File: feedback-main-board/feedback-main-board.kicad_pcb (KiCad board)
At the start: 4 copper layers, 80 x 64 mm, 88 parts, among them J1 908140508, J2 FLIP, J3 RPT, Q1 MMFTP3401, Q2 MMBT3904, Q3 MMBT3904, Q4 MMBT3904, SW1 SW_SPDT, SW2 SW_SPDT, U1 TL074, U2 TL074, U3 DG403, U4 NE555P, U5 4070

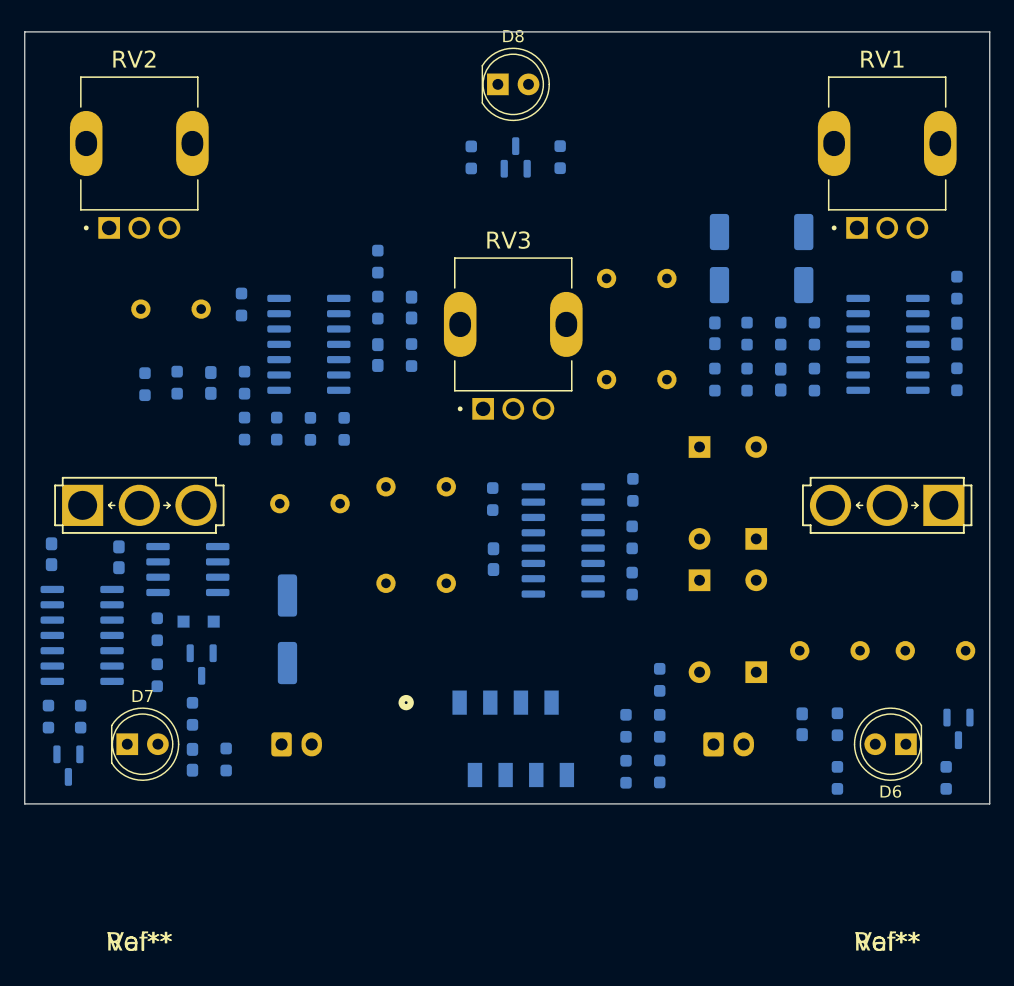
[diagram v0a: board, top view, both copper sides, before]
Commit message: Routing v1 done
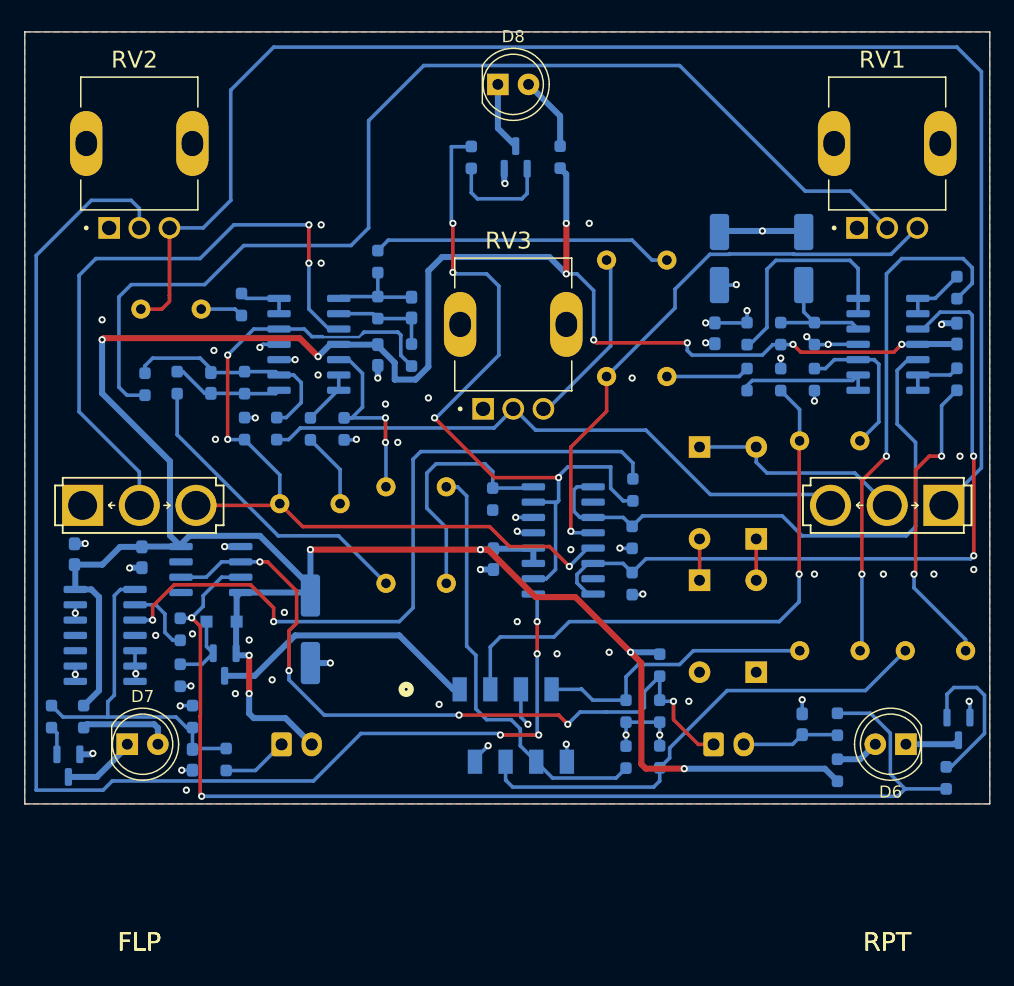
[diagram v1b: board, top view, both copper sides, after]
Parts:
- C5: footprint Capacitor_SMD:C_0603_1608Metric_Pad1.08x0.95mm_HandSolder -> Capacitor_THT:C_Rect_L7.0mm_W2.5mm_P5.00mm
- FLP: renamed from Ref**; value Val** -> FLP
- RPT: renamed from Ref**; value Val** -> RPT
- moved C13 9.91 mm to (112.7, 89.9)
- moved C7 9.54 mm to (112.7, 99.6), turned to 180 degrees
- moved C5 5.32 mm to (123.7, 104.9), turned to 0 degrees
- moved R5 2.79 mm to (122.2, 99.8)
- moved R9 2.67 mm to (119.4, 99.8)
- moved C1 1.91 mm to (83.2, 120.5)
- moved C17 1.91 mm to (69.2, 114.6)
- moved C22 1.91 mm to (63.6, 114.3)
- moved D1 1.91 mm to (75.8, 119.9)
- moved R1 1.91 mm to (72.4, 124.3)
- moved R30 1.91 mm to (72.4, 120.5)
- moved U4 1.91 mm to (74.9, 115.6)
- moved U5 1.91 mm to (66.2, 121.0)
- moved Q1 1.90 mm to (76.1, 123.4)
- moved R24 1.21 mm to (112.1, 123.5)
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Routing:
- net /+9V: track 0.00 -> 247.7 mm, vias 0 -> 14
- net /Core/OutPreVol: track 0.00 -> 125.7 mm
- net /Core/FxOut: track 0.00 -> 112.2 mm, vias 0 -> 4
- net /GND: track 0.00 -> 104.1 mm, vias 0 -> 58
- net /Switching/LatchState: track 0.00 -> 94.3 mm, vias 0 -> 2
- net /Core/InGain: track 0.00 -> 92.3 mm
- net /Core/RetBuf: track 0.00 -> 69.4 mm, vias 0 -> 3
- net /Switching/BypassState: track 0.00 -> 62.8 mm, vias 0 -> 4
- net /LatchSw1: track 0.00 -> 62.3 mm, vias 0 -> 5
- net Net-(R23-Pad2): track 0.00 -> 61.8 mm, vias 0 -> 2
- net Net-(R32-Pad2): track 0.00 -> 59.8 mm, vias 0 -> 2
- net Net-(SW1-Pad2): track 0.00 -> 52.1 mm, vias 0 -> 2
- net /Core/Feedback: track 0.00 -> 50.3 mm
- net Net-(R22-Pad2): track 0.00 -> 49.3 mm
- net /In: track 0.00 -> 48.8 mm, vias 0 -> 1
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- added copper zone on B.Cu, net /+4V5
- added copper zone on F.Cu, net /+4V5
- added copper zone on In1.Cu, net /GND
- added copper zone on In2.Cu, net /GND
